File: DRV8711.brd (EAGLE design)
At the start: 47.5 x 44.7 mm, 32 parts, among them IC1 DRV8711, T1 IPC50N04S5, T2 IPC50N04S5, T3 IPC50N04S5, T4 IPC50N04S5, T5 IPC50N04S5, T6 IPC50N04S5, T7 IPC50N04S5, T8 IPC50N04S5

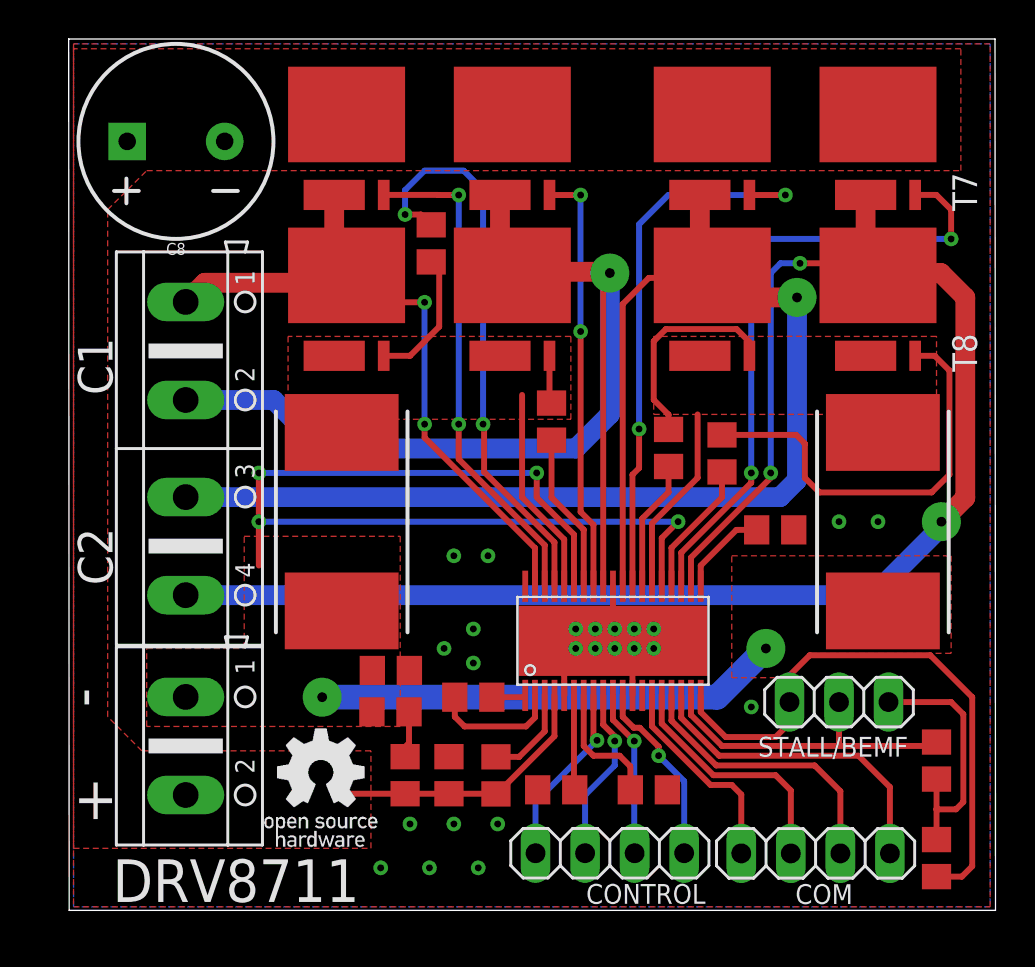
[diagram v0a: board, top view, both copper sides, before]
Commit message: Add files via upload
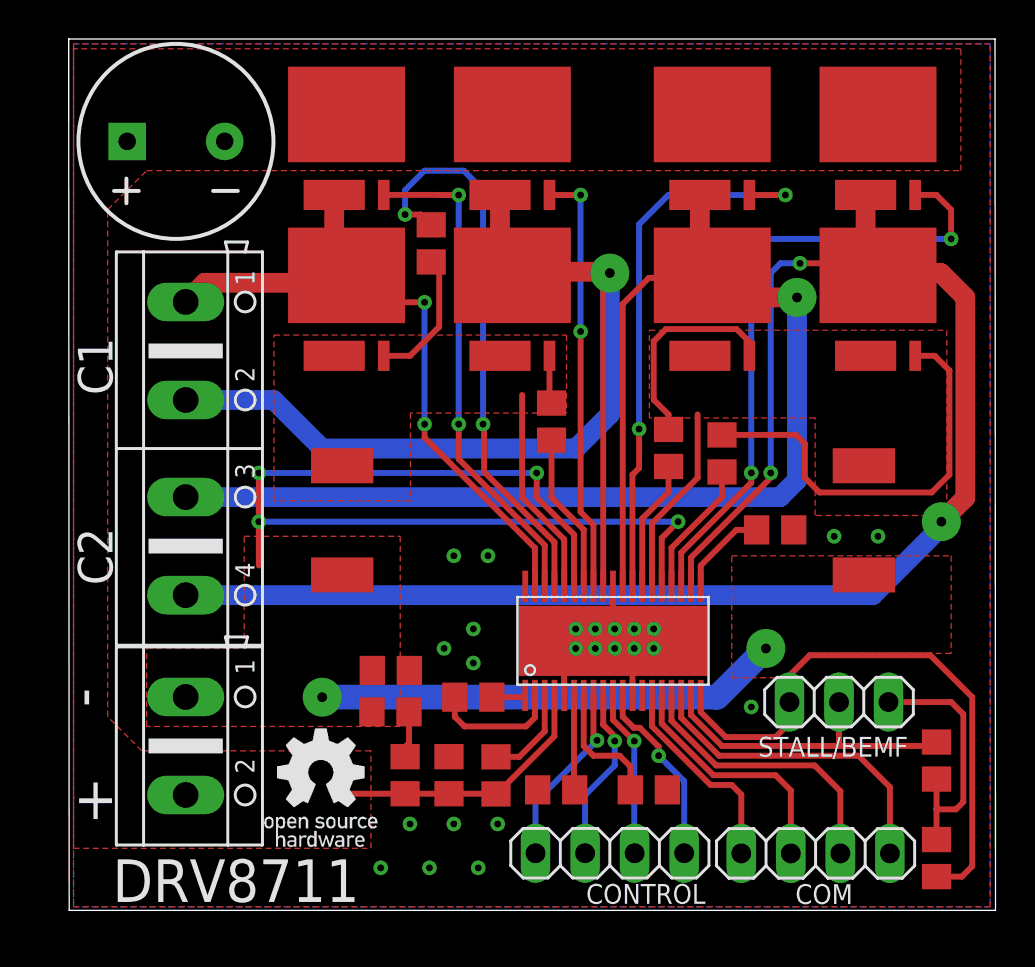
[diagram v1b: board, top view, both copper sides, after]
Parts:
- R1, R2: value 0.05R/5W -> 0.3R/2W; device rcl:R4527 -> rcl:R2512
- moved R2 0.98 mm to (40.8, 20.0)
- moved R1 0.07 mm to (14.0, 20.0)
